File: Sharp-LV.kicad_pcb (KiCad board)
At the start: 4 copper layers, 69.7 x 44.7 mm, 53 parts, among them J1 USB_C_Receptacle_USB2.0, J2 Conn_01x05_PROG, J3 5024260810, J4 FH52-10S-0.5SH_99, J5 SM04B-SRSS-TB_LF__SN_, J6 Conn_2Rows-13Pins, J7 S2B-PH-SM4-TB_LF__SN_, U1 NRF52840-QIAA-R, U2 USBLC6-2P6, U3 MCP1700-3302E_SOT23, U4 RT9080-33GJ5, U5 TPS2113APW, Y1 32.768K, Y2 Crystal 32Mhz, Y3 RV-3032-C7

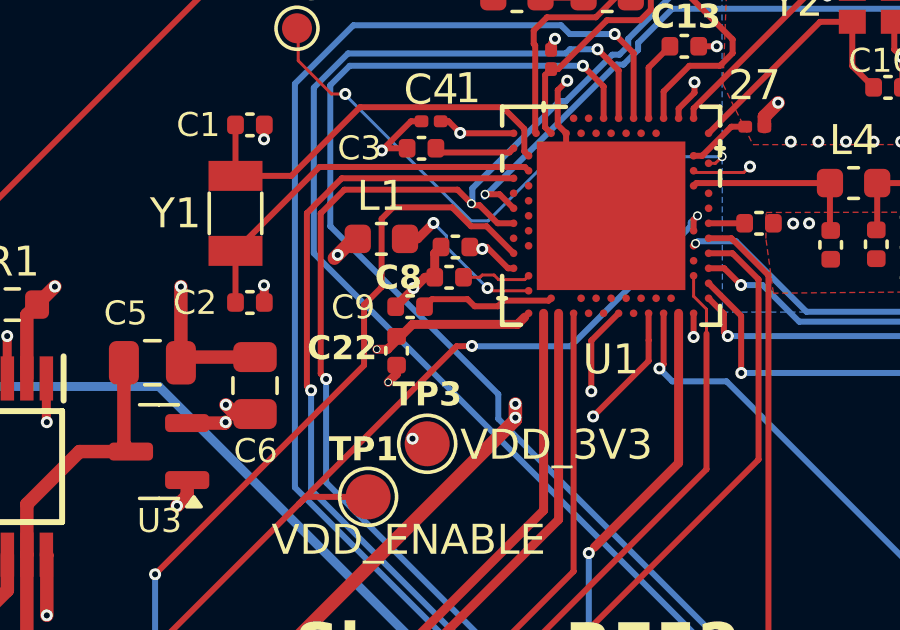
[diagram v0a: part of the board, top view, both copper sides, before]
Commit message: Update SCH & DRC
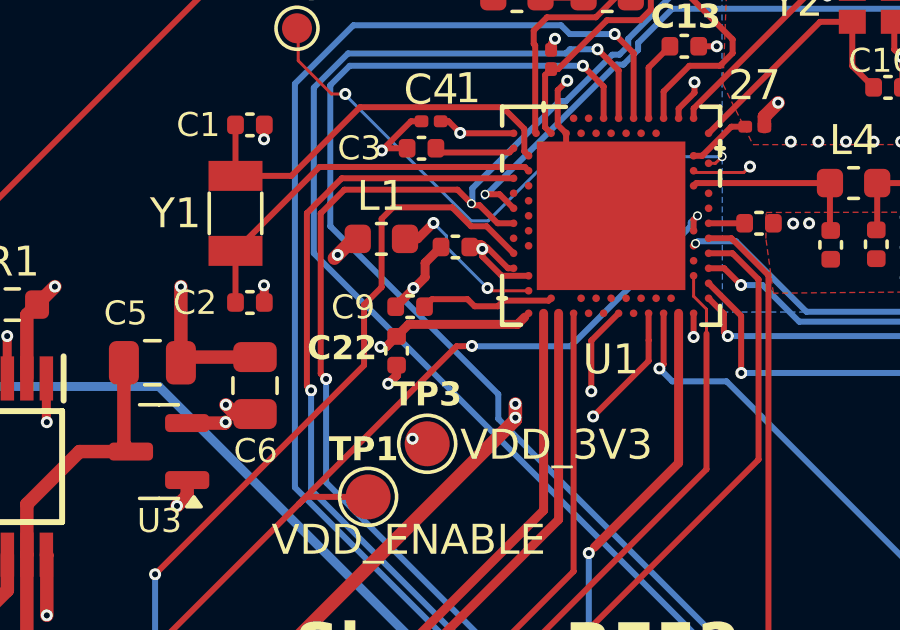
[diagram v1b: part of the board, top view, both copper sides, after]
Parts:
- removed C8: 4.7uF, Capacitor_SMD:C_0402_1005Metric
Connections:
- C7 pad 2: VDD2 -> VDD
- U1 pad W1: VDD2 -> VDD
- U1 pad Y2: Net-(U1-VDDH) -> VDD
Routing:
- net VDD: track 141.1 -> 149.8 mm, vias 9 -> 10
- net VDD2: track 153.7 -> 145.9 mm, vias 8 -> 7
- net Net-(U1-VDDH): track 2.32 -> 0.00 mm
